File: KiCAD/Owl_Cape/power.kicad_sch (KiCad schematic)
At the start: 16 parts, among them J22 9-16 In, J23 1-8 In, U2 D-SUN_MP1584_BUCK

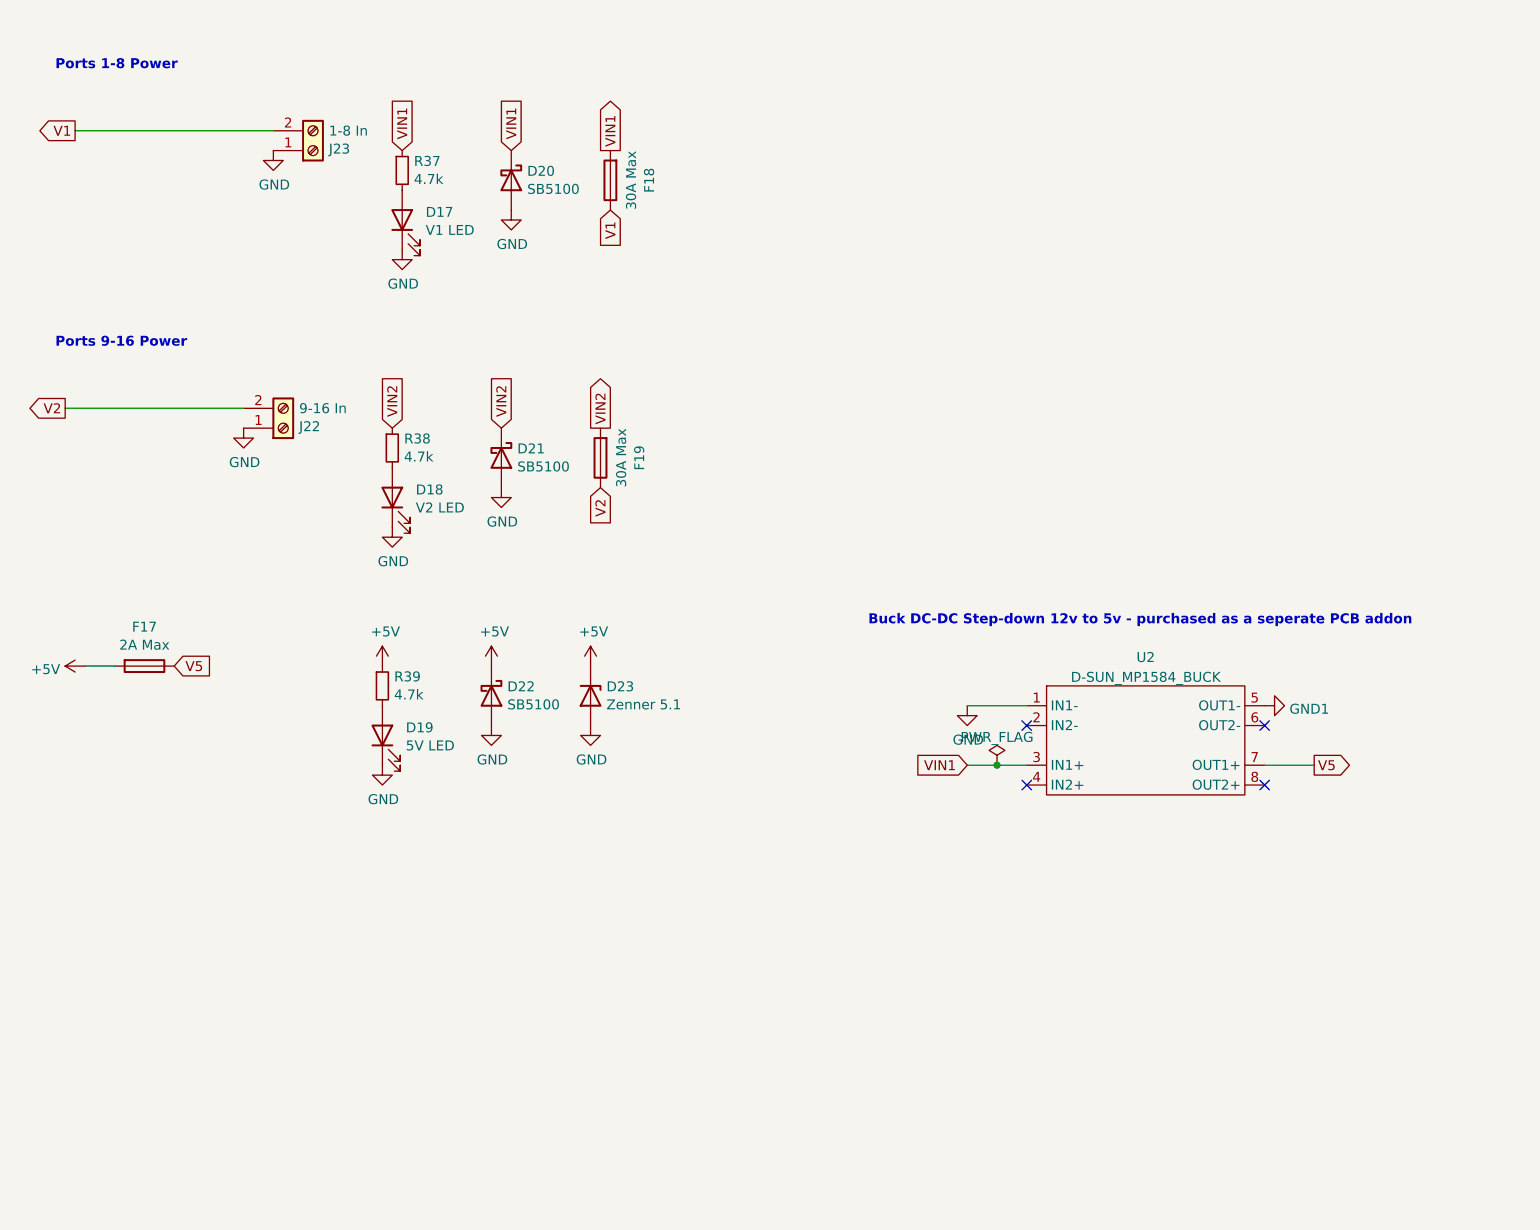
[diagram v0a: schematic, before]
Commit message: major update to layout
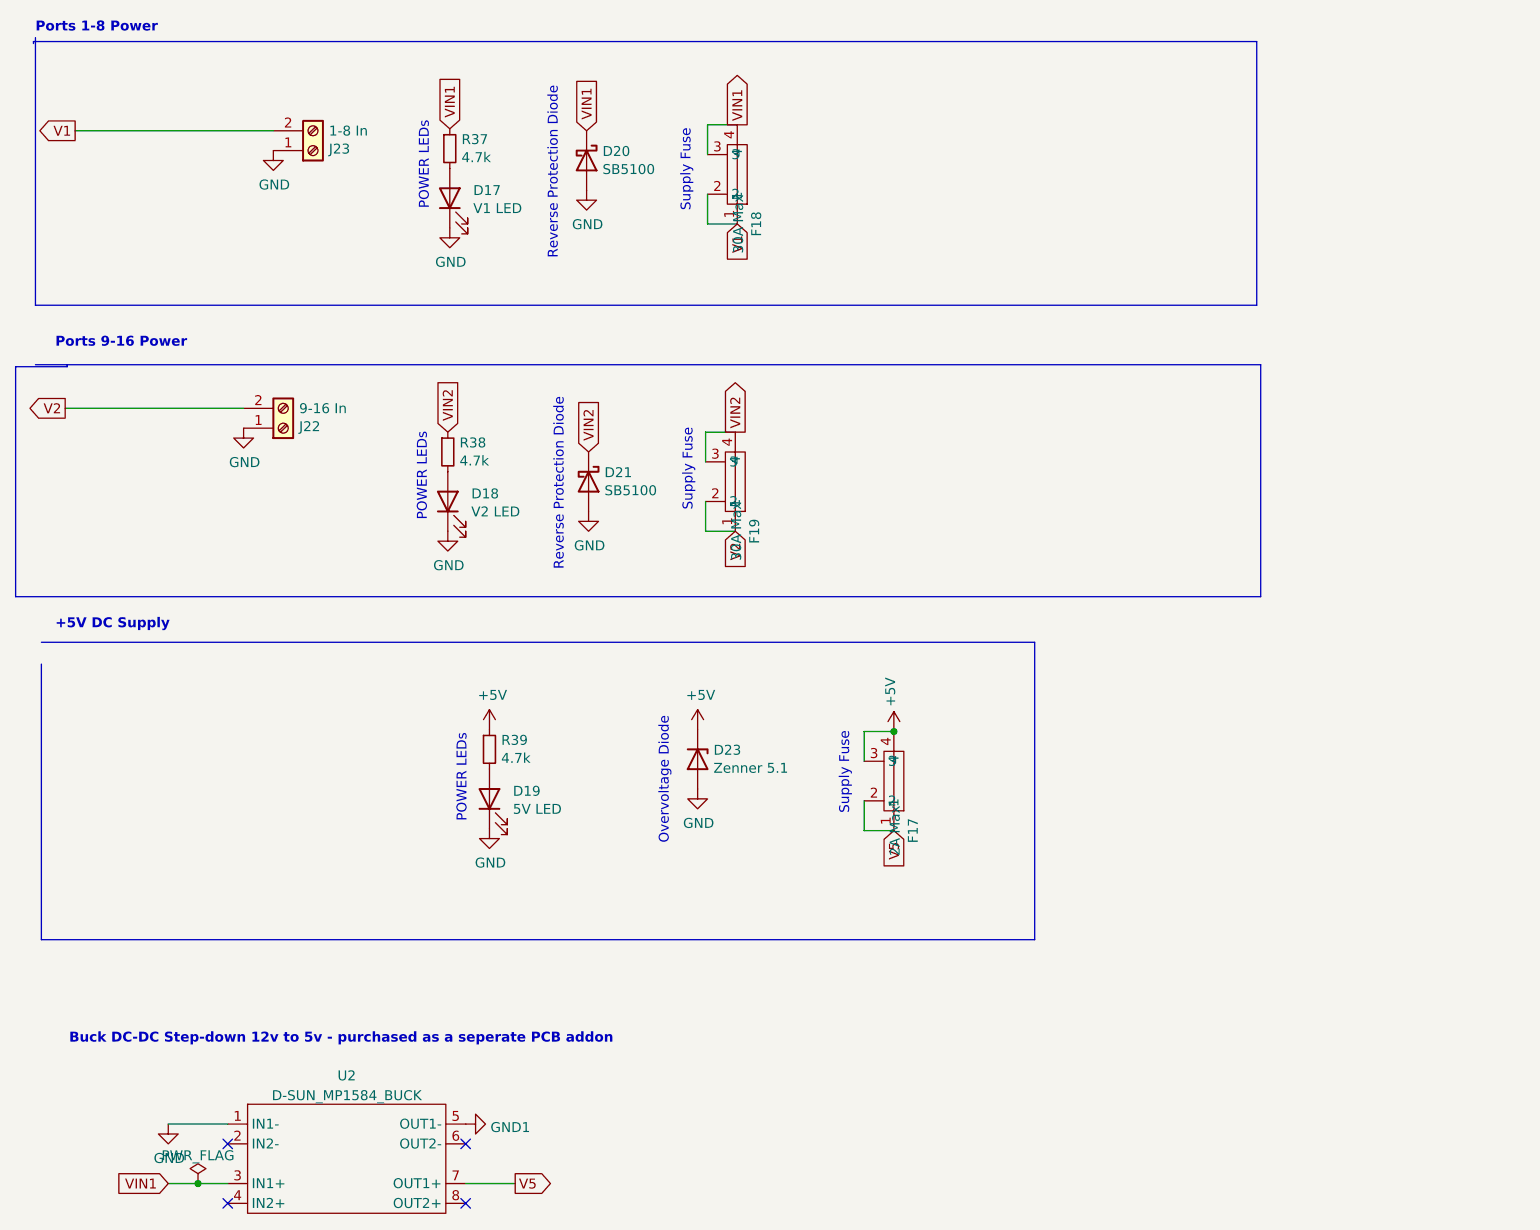
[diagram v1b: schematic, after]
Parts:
- removed D22: SB5100, Diode_THT:D_DO-201AD_P12.70mm_Horizontal, symbol Device:D_Schottky
- F17, F18, F19: footprint Fuse:Fuseholder_Blade_Mini_Keystone_3568 -> Stuart_BESPOKE:Medium Auto Fuse Holder; symbol Device:Fuse -> Stuarts_BESPOKE:Medium_Auto_Fuse_Holder
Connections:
- net +5V: now also F17.3, F17.4; no longer F17.2
- net V1: now also F18.2
- net V2: now also F19.2
- net V5: now also F17.2
- net VIN1: now also F18.3, F18.4; no longer F18.2
- net VIN2: now also F19.3, F19.4; no longer F19.2
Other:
- note added: "+5V DC Supply"
- note added: "Overvoltage Diode"
- note added: "POWER LEDs"
- note added: "Reverse Protection Diode"
- note added: "Supply Fuse"
- moved on the sheet: D17, D18, D19, D20, D21, D23, R37, R38, R39, U2
